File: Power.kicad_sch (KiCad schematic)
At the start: 90 parts, among them J10 Conn_01x02_Socket, J12 USB_C_Receptacle_USB2.0_14P, J22 Conn_01x02_Socket, J23 Conn_01x02_Socket, J24 Conn_01x02_Socket, J25 Conn_01x02_Socket, Q1 NMOS, Q6 NMOS, Q7 NMOS, U10 INA219AxD, U11 TLV62569ADRL, U12 USBLC6-2P6, U15 TPS60400DBV, U17 TCPP03-M20, U18 TPS54302, U4 TPS513885VABR, U9 INA219AxD

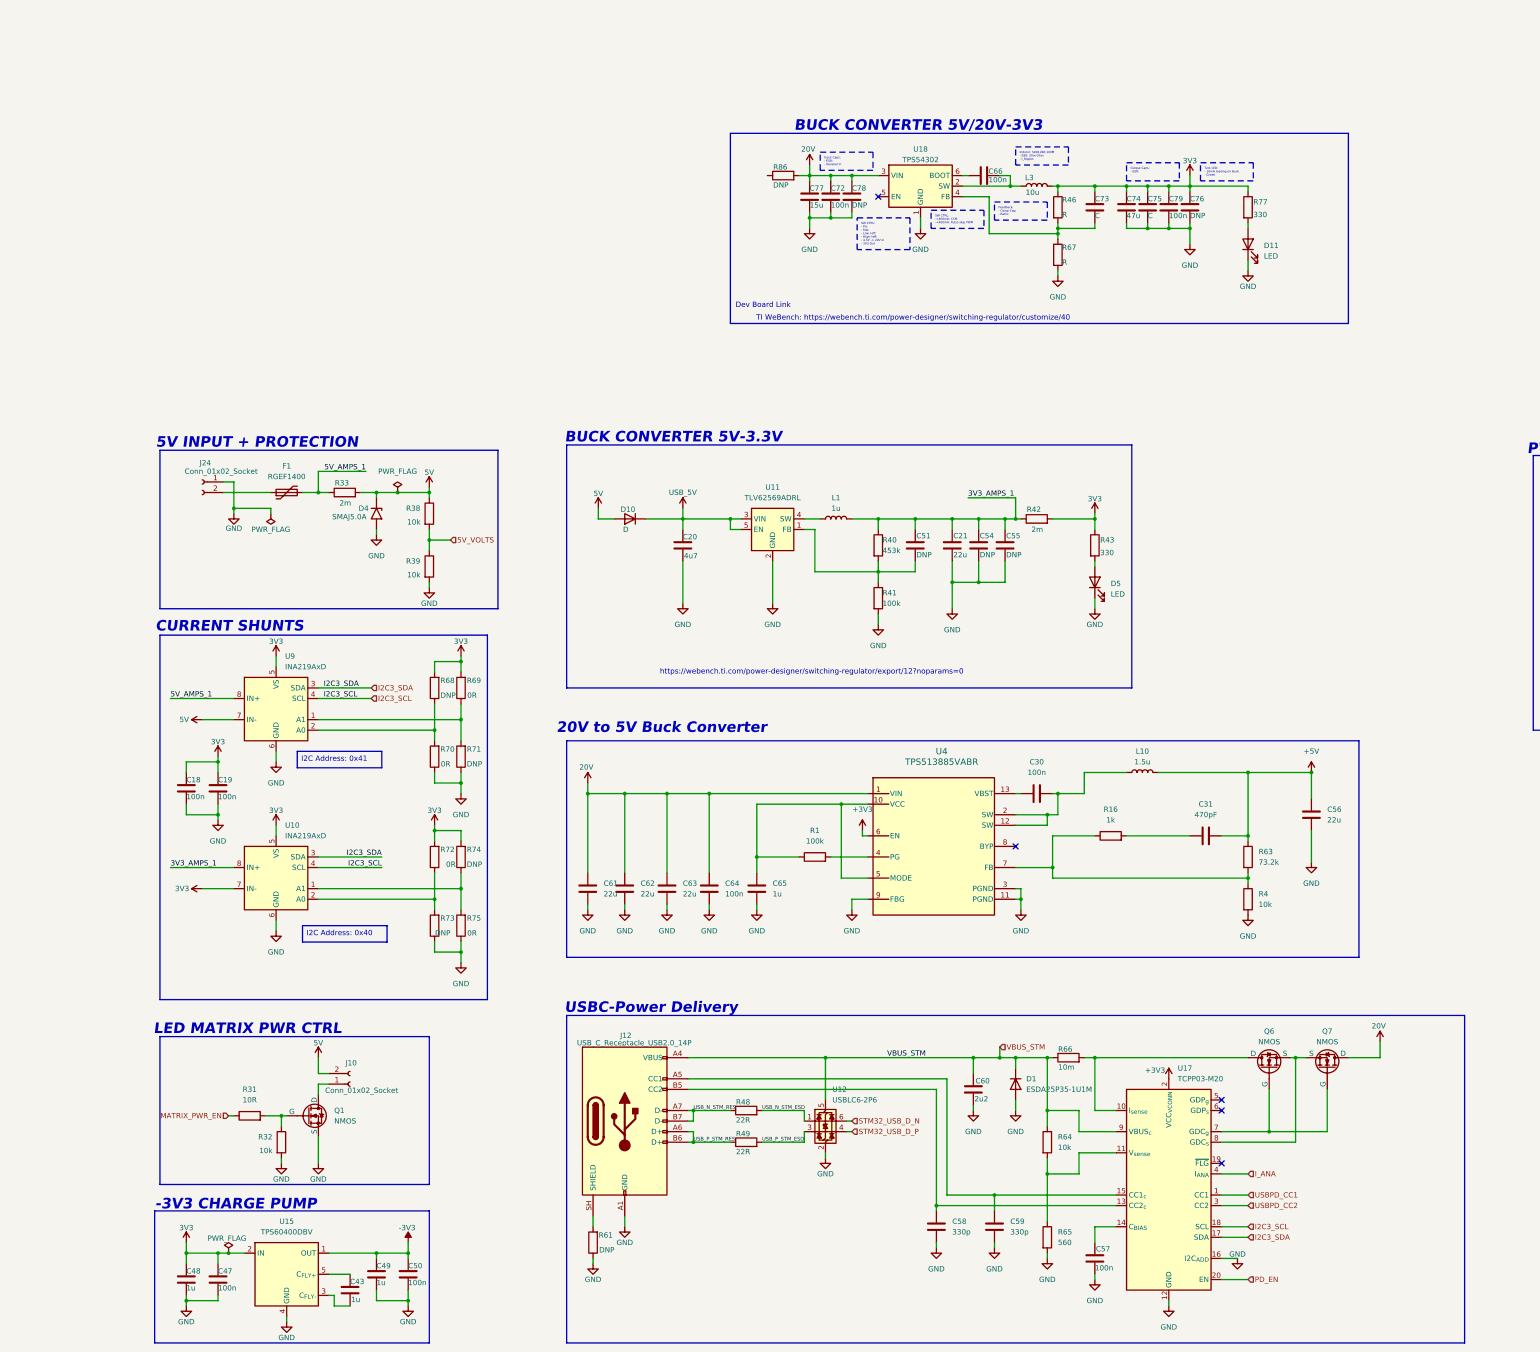
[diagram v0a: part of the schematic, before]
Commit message: PWR
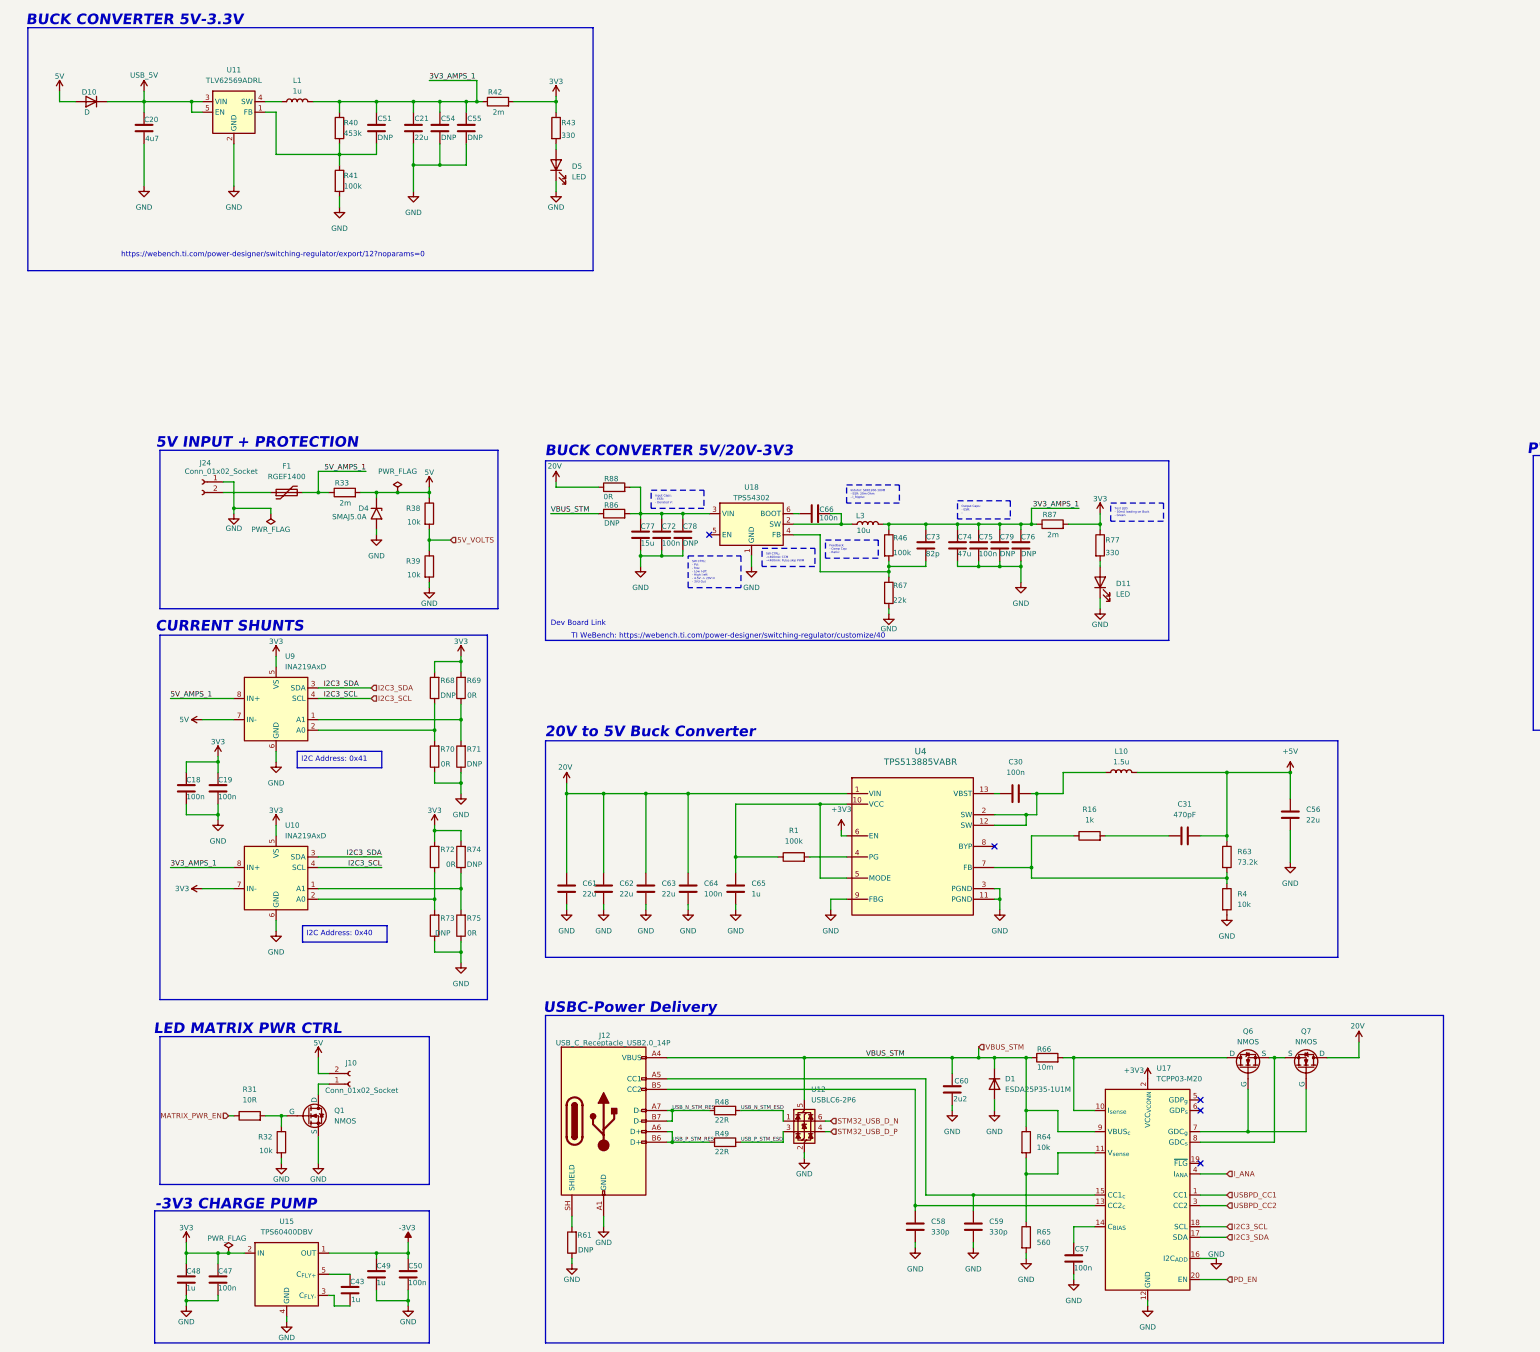
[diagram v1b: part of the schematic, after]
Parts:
- added R87: 2m, Resistor_SMD:R_0603_1608Metric, symbol Device:R
- added R88: 0R, Resistor_SMD:R_1210_3225Metric_Pad1.30x2.65mm_HandSolder, symbol Device:R
- C73: value C -> 82p
- C75: value C -> 100n
- C79: value 100n -> DNP
- R46: value R -> 100k
- R67: value R -> 22k
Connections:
- net 20V: now also R88.1; no longer C72.1, C77.1, C78.1, R86.2, U18.3 (VIN)
- net 3V3: now also R87.2; no longer C73.1, C74.1, C75.1, C76.1, C79.1, L3.2, R46.1
- net 3V3_AMPS_1: now also C73.1, C74.1, C75.1, C76.1, C79.1, L3.2, R46.1, R87.1
- net VBUS_STM: now also R86.1
- new net: C72.1, C77.1, C78.1, R86.2, R88.2, U18.3 (VIN)
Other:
- moved on the sheet: C20, C21, C30, C31, C51, C54, C55, C56, C57, C58, C59, C60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
